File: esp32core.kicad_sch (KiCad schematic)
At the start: 1 part

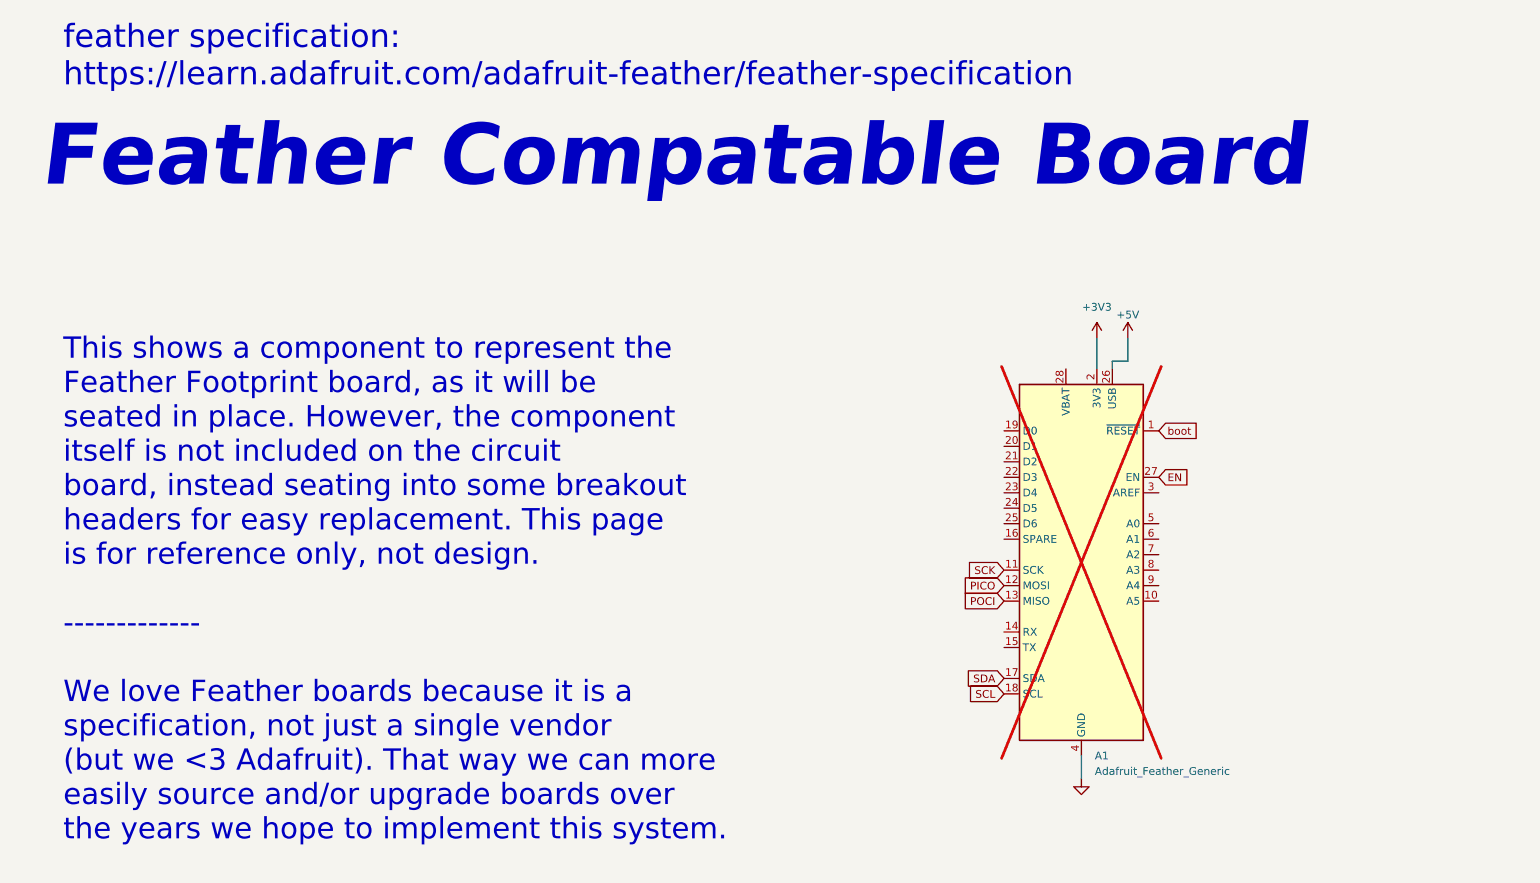
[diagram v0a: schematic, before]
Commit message: close enough for 3D export
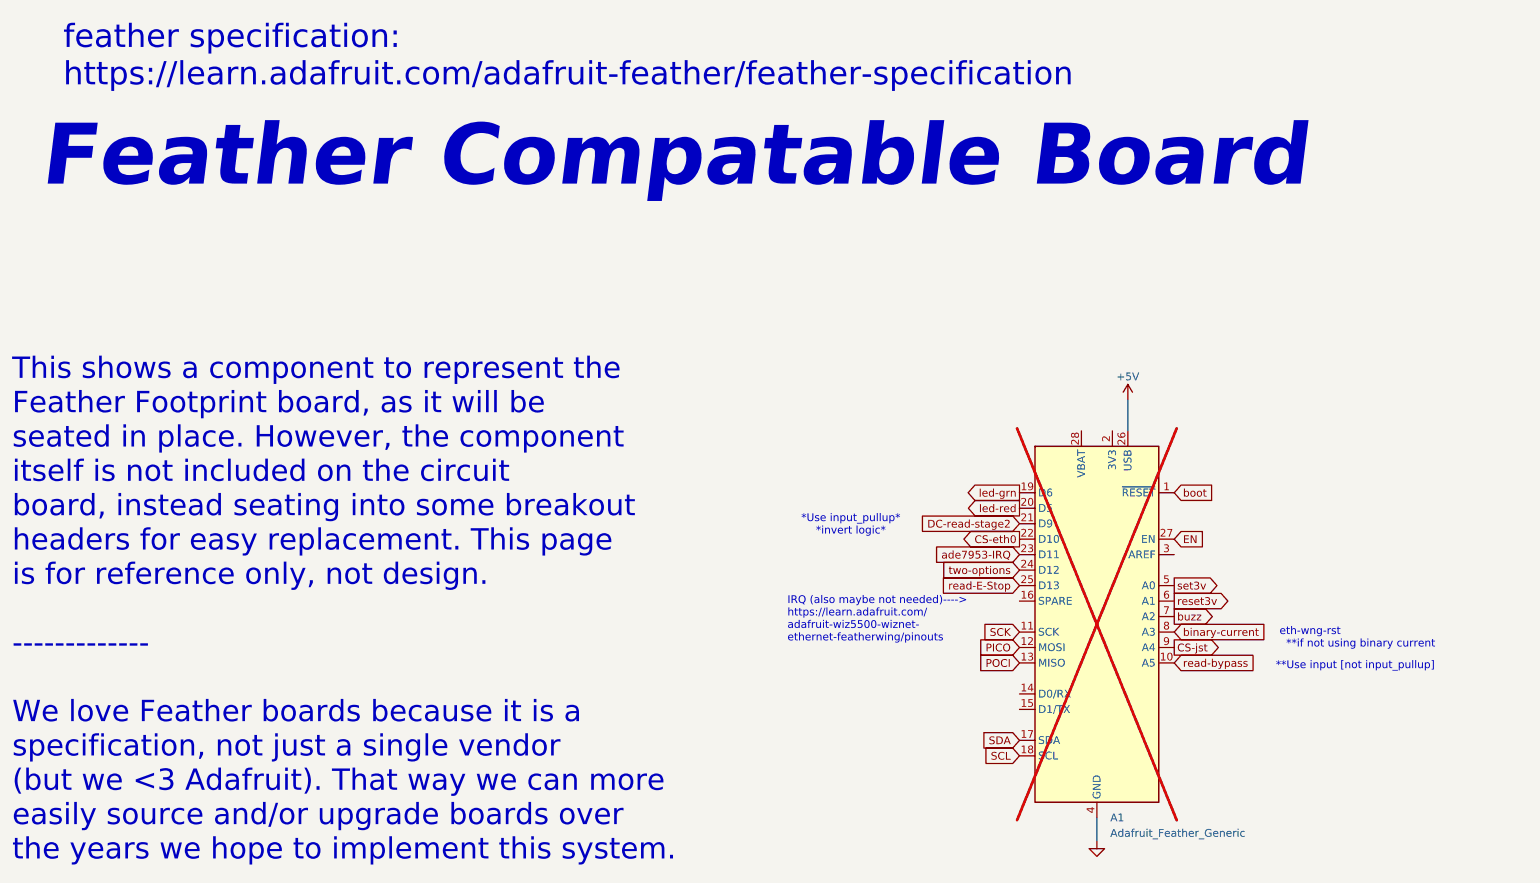
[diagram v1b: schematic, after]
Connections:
- net read-bypass: now reaches A1.10 (A5)
- net led-grn: now reaches A1.19 (D6)
- net led-red: now reaches A1.20 (D5)
- net DC-read-stage2: now reaches A1.21 (D9)
- net CS-eth0: now reaches A1.22 (D10)
- net ade7953-IRQ: now reaches A1.23 (D11)
- net two-options: now reaches A1.24 (D12)
- net read-E-Stop: now reaches A1.25 (D13)
- net set3v: now reaches A1.5 (A0)
- net reset3v: now reaches A1.6 (A1)
- net buzz: now reaches A1.7 (A2)
- net binary-current: now reaches A1.8 (A3)
- net CS-jst: now reaches A1.9 (A4)
- net +3V3: no longer names the net of A1.2 (3V3)
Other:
- note added: "**Use input [not input_pullup]"
- note added: "*Use input_pullup* *invert logic*"
- note added: "IRQ (also maybe not needed)----> https://learn.adafruit.com/ adafruit-wiz5500-wiznet- ethernet-featherwing/pinouts"
- note added: "eth-wng-rst **if not using binary current"
- moved on the sheet: A1
